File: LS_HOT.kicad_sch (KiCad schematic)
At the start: 3 parts, among them U6 VNLD5160TR-E

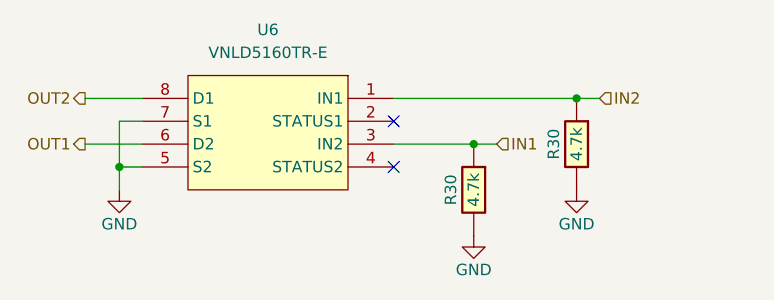
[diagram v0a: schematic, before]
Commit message: Unification with UAEFI F7 #114 #110
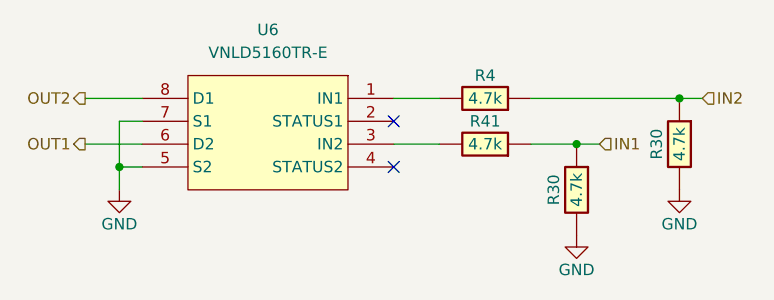
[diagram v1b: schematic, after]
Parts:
- added R4, R41: 4.7k, hellen-one-common:R0603, symbol hellen-one-common:Res
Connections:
- net IN1: now also R41.1; no longer U6.3 (IN2)
- net IN2: now also R4.1; no longer U6.1 (IN1)
- new net: R4.2, U6.1 (IN1)
- new net: R41.2, U6.3 (IN2)
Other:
- moved on the sheet: R30
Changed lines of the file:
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@@
 	(title_block
 		(title "UAEFI")
-		(date "2025-04-30")
-		(rev "E")
+		(date "2026-07-05")
+		(rev "F")
 		(company "rusEFI.com")
 	)
 	(junction
-		(at 168.91 91.44)
+		(at 180.34 91.44)
 		(diameter 0)
 		(color 0 0 0 0)
@@
 	)
 	(junction
-		(at 180.34 86.36)
+		(at 191.77 86.36)
 		(diameter 0)
 		(color 0 0 0 0)
@@
 	(wire
 		(pts
-			(xy 168.91 91.44) (xy 171.45 91.44)
-		)
-		(stroke
-			(width 0)
-			(type default)
-		)
-	)
-	(wire
-		(pts
-			(xy 160.02 86.36) (xy 180.34 86.36)
-		)
-		(stroke
-			(width 0)
-			(type default)
-		)
-	)
-	(wire
-		(pts
-			(xy 160.02 91.44) (xy 168.91 91.44)
+			(xy 180.34 91.44) (xy 182.88 91.44)
+		)
+		(stroke
+			(width 0)
+			(type default)
+		)
+	)
+	(wire
+		(pts
+			(xy 160.02 86.36) (xy 165.1 86.36)
+		)
+		(stroke
+			(width 0)
+			(type default)
+		)
+	)
+	(wire
+		(pts
+			(xy 175.26 91.44) (xy 180.34 91.44)
+		)
+		(stroke
+			(width 0)
+			(type default)
+		)
+	)
+	(wire
+		(pts
+			(xy 160.02 91.44) (xy 165.1 91.44)
 		)
 		(stroke
@@
 	(wire
 		(pts
+			(xy 175.26 86.36) (xy 191.77 86.36)
+		)
+		(stroke
+			(width 0)
+			(type default)
+		)
+	)
+	(wire
+		(pts
 			(xy 129.54 96.52) (xy 129.54 93.98)
 		)
@@
 	(wire
 		(pts
-			(xy 180.34 86.36) (xy 182.88 86.36)
+			(xy 191.77 86.36) (xy 194.31 86.36)
 		)
 		(stroke
@@
 	(hierarchical_label "IN2"
 		(shape input)
-		(at 182.88 86.36 0)
+		(at 194.31 86.36 0)
 		(effects
 			(font
@@
 	(hierarchical_label "IN1"
 		(shape input)
-		(at 171.45 91.44 0)
+		(at 182.88 91.44 0)
 		(effects
 			(font
@@
 	(symbol
 		(lib_id "power:GND")
-		(at 180.34 96.52 0)
+		(at 191.77 96.52 0)
 		(unit 1)
 		(exclude_from_sim no)
@@
 		(dnp no)
 		(property "Reference" "#PWR035"
-			(at 180.34 102.87 0)
+			(at 191.77 102.87 0)
 			(effects
 				(font
@@
 		)
 		(property "Value" "GND"
-			(at 180.34 100.33 0)
+			(at 191.77 100.33 0)
 			(effects
 				(font
@@
 		)
 		(property "Footprint" ""
-			(at 180.34 96.52 0)
+			(at 191.77 96.52 0)
 			(effects
 				(font
@@
 		)
 		(property "Datasheet" ""
-			(at 180.34 96.52 0)
+			(at 191.77 96.52 0)
 			(effects
 				(font
@@
 		)
 		(property "Description" "Power symbol creates a global label with name \"GND\" , ground"
-			(at 180.34 96.52 0)
+			(at 191.77 96.52 0)
 			(effects
 				(font
@@
 	(symbol
 		(lib_id "power:GND")
-		(at 168.91 101.6 0)
+		(at 180.34 101.6 0)
 		(unit 1)
 		(exclude_from_sim no)
@@
 		(dnp no)
 		(property "Reference" "#PWR035"
-			(at 168.91 107.95 0)
+			(at 180.34 107.95 0)
 			(effects
 				(font
@@
 		)
 		(property "Value" "GND"
-			(at 168.91 105.41 0)
+			(at 180.34 105.41 0)
 			(effects
 				(font
@@
 		)
 		(property "Footprint" ""
-			(at 168.91 101.6 0)
+			(at 180.34 101.6 0)
 			(effects
 				(font
@@
 		)
 		(property "Datasheet" ""
-			(at 168.91 101.6 0)
+			(at 180.34 101.6 0)
 			(effects
 				(font
@@
 		)
 		(property "Description" "Power symbol creates a global label with name \"GND\" , ground"
-			(at 168.91 101.6 0)
+			(at 180.34 101.6 0)
 			(effects
 				(font
@@
 	(symbol
 		(lib_id "hellen-one-common:Res")
-		(at 180.34 86.36 90)
+		(at 191.77 86.36 90)
 		(mirror x)
 		(unit 1)
@@
 		(dnp no)
 		(property "Reference" "R30"
-			(at 177.8 91.44 0)
+			(at 189.23 91.44 0)
 			(effects
 				(font
@@
 		)
 		(property "Value" "4.7k"
-			(at 180.34 91.44 0)
+			(at 191.77 91.44 0)
 			(effects
 				(font
@@
 		)
 		(property "Footprint" "hellen-one-common:R0603"
-			(at 184.15 90.17 0)
+			(at 195.58 90.17 0)
 			(effects
 				(font
@@
 		)
 		(property "Datasheet" ""
-			(at 180.34 86.36 0)
+			(at 191.77 86.36 0)
 			(effects
 				(font
@@
 		)
 		(property "Description" ""
-			(at 180.34 86.36 0)
+			(at 191.77 86.36 0)
 			(effects
 				(font
@@
 		)
 		(property "LCSC" "C23162"
-			(at 180.34 86.36 0)
+			(at 191.77 86.36 0)
 			(effects
 				(font
@@
 	(symbol
 		(lib_id "hellen-one-common:Res")
-		(at 168.91 91.44 90)
+		(at 175.26 91.44 0)
+		(mirror y)
+		(unit 1)
+		(exclude_from_sim no)
+		(in_bom yes)
+		(on_board yes)
+		(dnp no)
+		(property "Reference" "R41"
+			(at 170.18 88.9 0)
+			(effects
+				(font
+					(size 1.27 1.27)
+				)
+			)
+		)
+		(property "Value" "4.7k"
+			(at 170.18 91.44 0)
+			(effects
+				(font
+					(size 1.27 1.27)
+				)
+			)
+		)
+		(property "Footprint" "hellen-one-common:R0603"
+			(at 171.45 95.25 0)
+			(effects
+				(font
+					(size 1.27 1.27)
+				)
+				(hide yes)
+			)
+		)
+		(property "Datasheet" ""
+			(at 175.26 91.44 0)
+			(effects
+				(font
+					(size 1.27 1.27)
+				)
+				(hide yes)
+			)
+		)
+		(property "Description" ""
+			(at 175.26 91.44 0)
+			(effects
+				(font
+					(size 1.27 1.27)
+				)
+				(hide yes)
+			)
+		)
+		(property "LCSC" "C23162"
+			(at 175.26 91.44 0)
+			(effects
+				(font
+					(size 1.27 1.27)
+				)
+				(hide yes)
+			)
+		)
+		(pin "1"
+		)
+		(pin "2"
+		)
+		(instances
+			(project "uaefi-pro"
+				(path "/ac264c30-3e9a-4be2-b97a-9949b68bd497/c1e0fc38-44a5-4f4c-8a40-7ced112340c0"
+					(reference "R41")
+					(unit 1)
+				)
+			)
+		)
+	)
+	(symbol
+		(lib_id "hellen-one-common:Res")
+		(at 180.34 91.44 90)
 		(mirror x)
 		(unit 1)
@@
 		(dnp no)
 		(property "Reference" "R30"
-			(at 166.37 96.52 0)
+			(at 177.8 96.52 0)
 			(effects
 				(font
@@
 		)
 		(property "Value" "4.7k"
-			(at 168.91 96.52 0)
+			(at 180.34 96.52 0)
 			(effects
 				(font
@@
 		)
 		(property "Footprint" "hellen-one-common:R0603"
-			(at 172.72 95.25 0)
+			(at 184.15 95.25 0)
 			(effects
 				(font
@@
 		)
 		(property "Datasheet" ""
-			(at 168.91 91.44 0)
+			(at 180.34 91.44 0)
 			(effects
 				(font
@@
 		)
 		(property "Description" ""
-			(at 168.91 91.44 0)
+			(at 180.34 91.44 0)
 			(effects
 				(font
@@
 		)
 		(property "LCSC" "C23162"
-			(at 168.91 91.44 0)
+			(at 180.34 91.44 0)
 			(effects
 				(font
@@
 					(unit 1)
 				)
+			)
+		)
+	)
+	(symbol
+		(lib_id "hellen-one-common:Res")
+		(at 175.26 86.36 0)
+		(mirror y)
+		(unit 1)
+		(exclude_from_sim no)
+		(in_bom yes)
+		(on_board yes)
+		(dnp no)
+		(property "Reference" "R4"
+			(at 170.18 83.82 0)
+			(effects
+				(font
+					(size 1.27 1.27)
+				)
+			)
+		)
+		(property "Value" "4.7k"
+			(at 170.18 86.36 0)
+			(effects
+				(font
+					(size 1.27 1.27)
+				)
+			)
+		)
+		(property "Footprint" "hellen-one-common:R0603"
+			(at 171.45 90.17 0)
+			(effects
+				(font
+					(size 1.27 1.27)
+				)
+				(hide yes)
+			)
+		)
+		(property "Datasheet" ""
+			(at 175.26 86.36 0)
+			(effects
+				(font
+					(size 1.27 1.27)
+				)
+				(hide yes)
+			)
+		)
+		(property "Description" ""
+			(at 175.26 86.36 0)
+			(effects
+				(font
+					(size 1.27 1.27)
+				)
+				(hide yes)
+			)
+		)
+		(property "LCSC" "C23162"
+			(at 175.26 86.36 0)
+			(effects
+				(font
+					(size 1.27 1.27)
+				)
+				(hide yes)
+			)
+		)
+		(pin "1"
+		)
+		(pin "2"
+		)
+		(instances
+			(project "uaefi-pro"
+				(path "/ac264c30-3e9a-4be2-b97a-9949b68bd497/c1e0fc38-44a5-4f4c-8a40-7ced112340c0"
+					(reference "R4")
+					(unit 1)
+				)
